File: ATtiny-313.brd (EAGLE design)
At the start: 27.6 x 64.1 mm, 15 parts

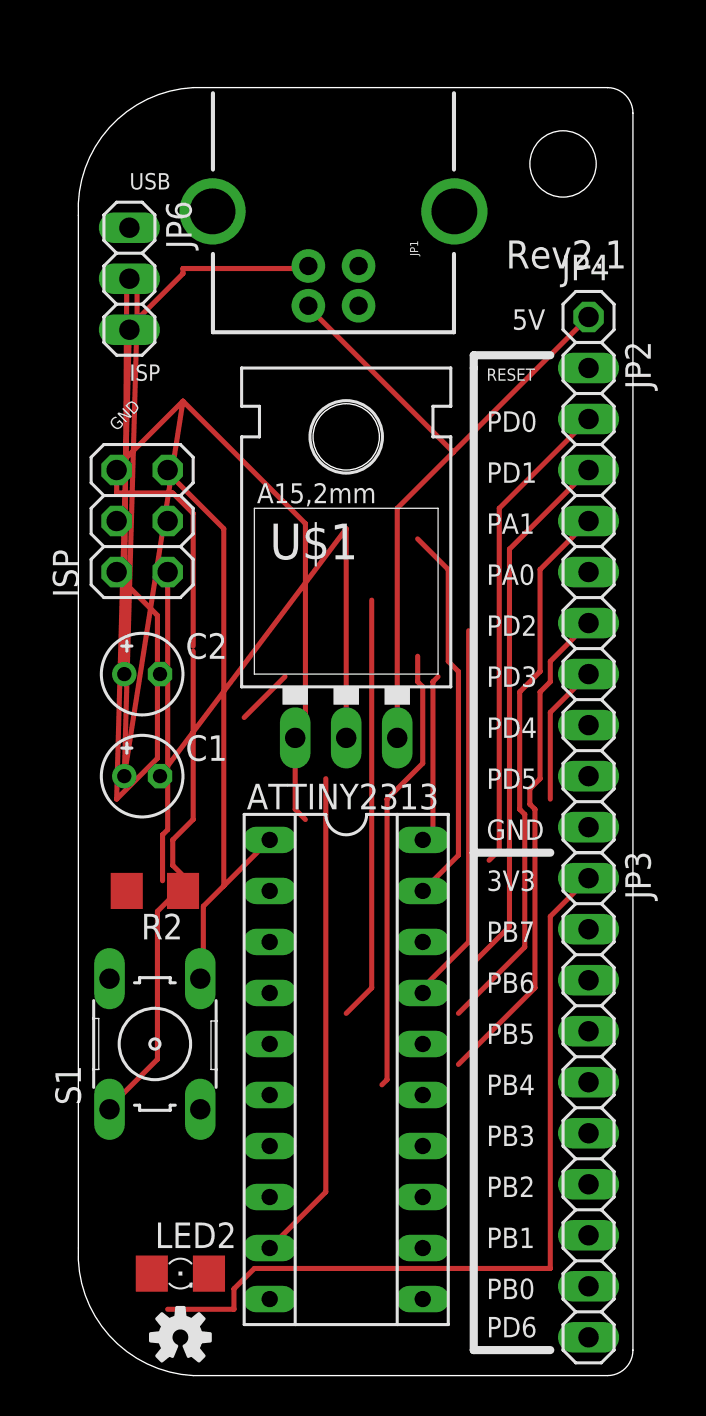
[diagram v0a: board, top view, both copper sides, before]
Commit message: more SMD goodness
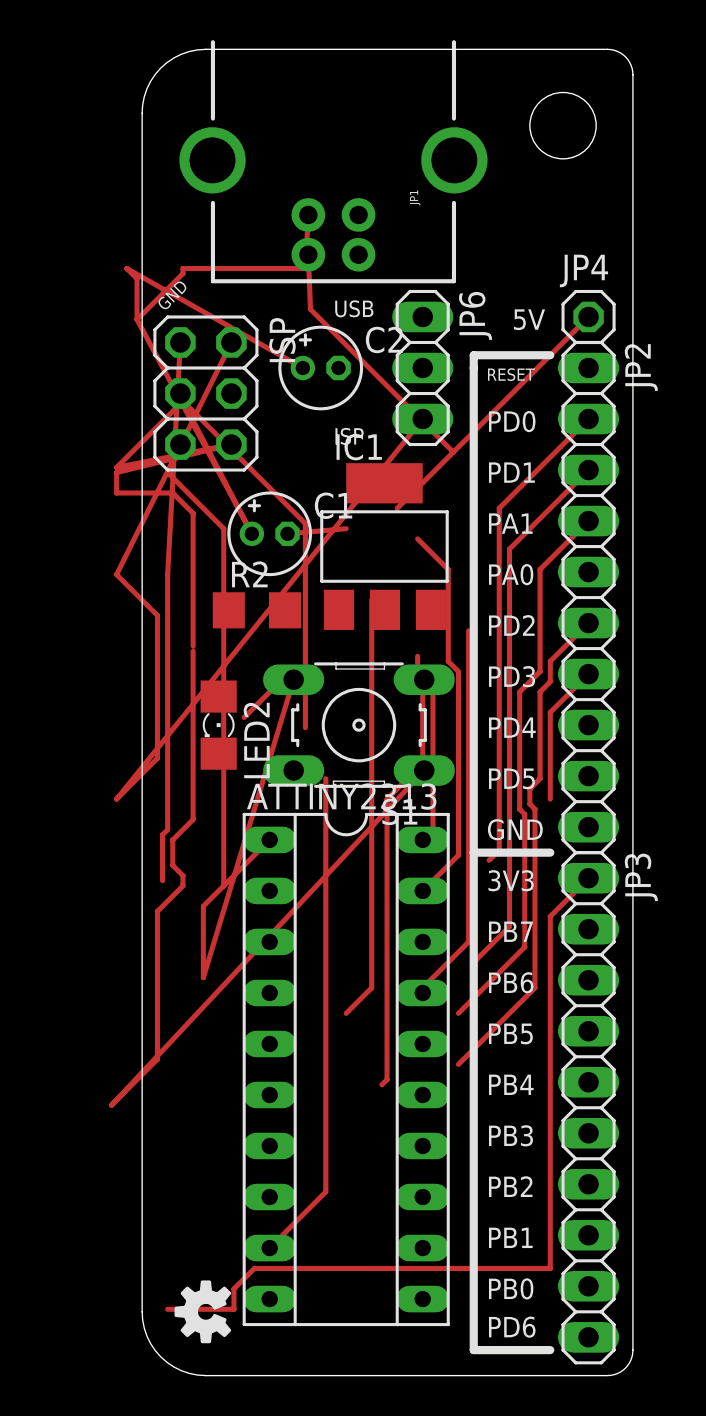
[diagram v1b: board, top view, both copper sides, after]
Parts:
- removed U$1: V_REG_LD1117VXX, SparkFun-PowerIC:78XXL
- added IC1: REG1117, burr-brown:SOT223
- moved LED2 27.4 mm to (19.1, 40.0), turned to 270 degrees
- moved S1 18.8 mm to (26.0, 40.0), turned to 180 degrees
- moved C2 17.6 mm to (24.1, 57.8)
- moved JP6 15.3 mm to (29.2, 57.8)
- moved R2 14.9 mm to (21.0, 45.7), turned to 0 degrees
- moved C1 13.6 mm to (21.6, 49.5)
- moved ISP 7.10 mm to (18.4, 56.5), turned to 270 degrees
- moved JP1 2.54 mm to (24.8, 65.4)
- moved U$2 1.91 mm to (36.2, 69.8)
- moved U$3 1.80 mm to (18.4, 10.8), turned to 90 degrees
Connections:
- net N$1: now also IC1.3; no longer U$1.OUT
- net N$3: now also IC1.1; no longer U$1.IN
- net N$4: now also IC1.2; no longer U$1.GND
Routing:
- net N$4: track 25.8 -> 2.93 mm
- net N$5: track 30.2 -> 47.0 mm
- net N$23: track 36.4 -> 50.0 mm
- net ISP: track 15.5 -> 26.9 mm
- net N$1: track 35.2 -> 26.2 mm
- net N$3: track 139.8 -> 139.1 mm
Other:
- board size 27.6 x 64.1 mm -> 24.4 x 66 mm
